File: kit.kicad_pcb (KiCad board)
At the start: 4 copper layers, 15 x 11.5 mm, 68 parts, among them IC1 TPA6130A2RTJR, J1 SJ-43617-SMT-TR, J2 Conn_01x06, U1 ESP32-S3-WROOM-1, U2 PCM5100A, U3 MIC5504-3.3YM5

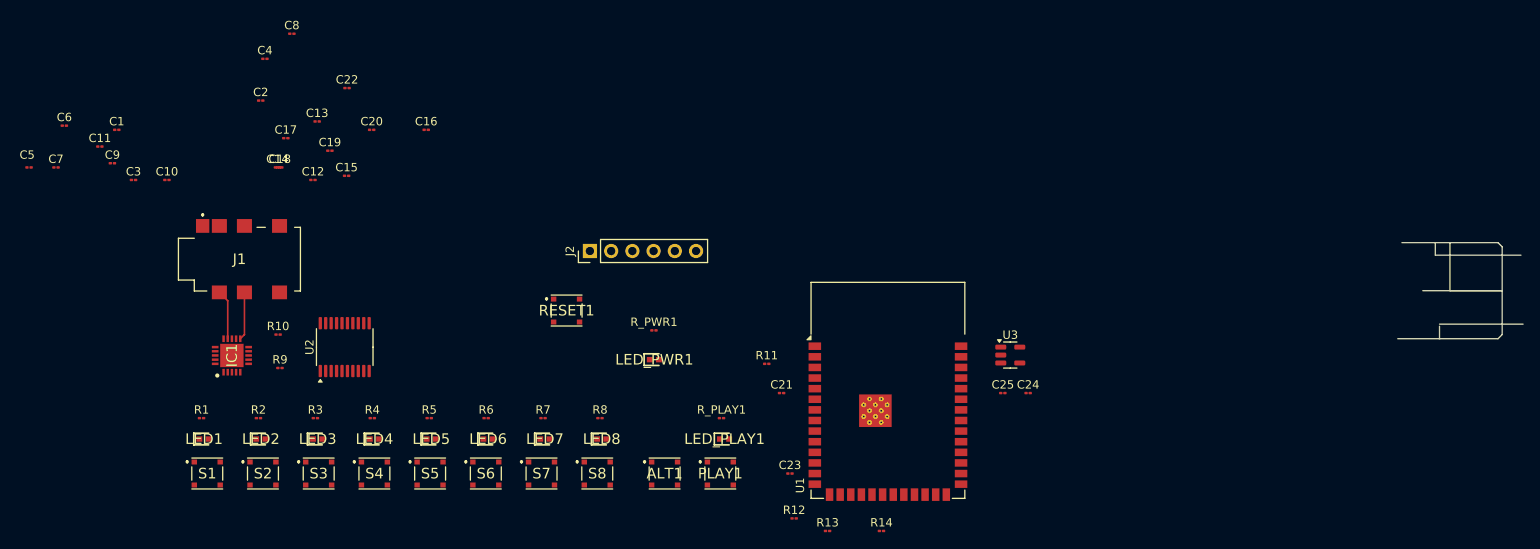
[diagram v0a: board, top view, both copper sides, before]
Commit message: Updates
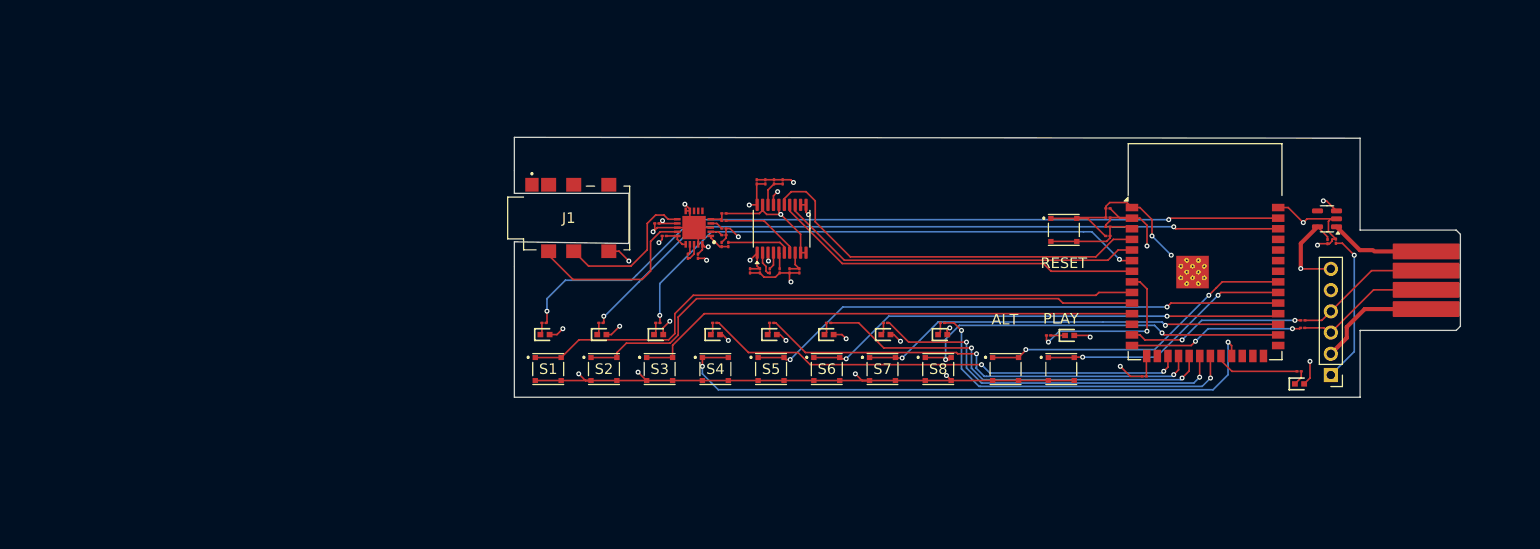
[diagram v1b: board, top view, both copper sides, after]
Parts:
- removed C11, C8: 0.47uF, Capacitor_SMD:C_01005_0402Metric
- moved C22 92.8 mm to (149.8, 40.7)
- moved J2 89.9 mm to (176.5, 57.3), turned to 180 degrees
- moved C5 80.7 mm to (100.8, 43.1), turned to -90 degrees
- moved R_PWR1 77.4 mm to (172.7, 56.9)
- moved LED_PWR1 77.3 mm to (172.8, 58.4)
- moved C6 76.2 mm to (99.6, 43.1), turned to 90 degrees
- moved C9 73.7 mm to (103.9, 40.6), turned to 180 degrees
- moved C7 72.2 mm to (95.8, 39.2), turned to 180 degrees
- moved C3 70.8 mm to (103.6, 41.7), turned to -90 degrees
- moved C10 66.9 mm to (103.9, 39.8), turned to 180 degrees
- moved C1 66.7 mm to (96.7, 40.7)
- moved C4 65.5 mm to (109.4, 44.9), turned to 90 degrees
- moved R12 65.3 mm to (173.2, 50.8)
- moved R13 61.8 mm to (173.1, 51.7)
- moved C14 60.5 mm to (110.9, 34.2), turned to -90 degrees
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- renumbered ALT1 to ALT, PLAY1 to PLAY, RESET1 to RESET
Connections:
- ALT pad 1: /SW_PLAY -> /SW_ALT
- ALT pad 3: /SW_PLAY -> /SW_ALT
- C2 pad 1: Net-(C11-Pad1) -> Net-(IC1-RIGHTINM)
- C3 pad 2: Net-(C3-Pad2) -> Net-(IC1-LEFTINM)
- J2 pad 3: /USB_DN -> /USB_DP
- J2 pad 4: /USB_DP -> /USB_DN
- PLAY pad 1: /SW_ALT -> /SW_PLAY
- PLAY pad 3: /SW_ALT -> /SW_PLAY
- R10 pad 2: Net-(C11-Pad1) -> Net-(IC1-RIGHTINM)
- R9 pad 2: Net-(C3-Pad2) -> Net-(IC1-LEFTINM)
- U1 pad 28: /SW_5 -> /SW_8
- U1 pad 29: /SW_6 -> /SW_7
- U1 pad 30: /SW_7 -> /SW_6
- U1 pad 31: /SW_8 -> /SW_5
- U1 pad 7: /LCM_DIN -> /PCM_DIN
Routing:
- net GND: track 0.00 -> 199.9 mm, vias 0 -> 19
- net +5V: track 0.00 -> 138.7 mm, vias 0 -> 4
- net /LED_1: track 0.00 -> 94.6 mm, vias 0 -> 2
- net /LED_2: track 0.00 -> 86.1 mm, vias 0 -> 2
- net /SW_1: track 0.00 -> 76.0 mm
- net /SW_4: track 0.00 -> 75.2 mm, vias 0 -> 2
- net /SW_2: track 0.00 -> 69.5 mm
- net /LED_3: track 0.00 -> 65.2 mm, vias 0 -> 2
- net /SW_5: track 0.00 -> 65.1 mm, vias 0 -> 2
- net /SW_3: track 0.00 -> 61.1 mm
- net +3.3V: track 0.00 -> 58.8 mm, vias 0 -> 16
- net /LED_4: track 0.00 -> 58.1 mm, vias 0 -> 2
- net /SW_6: track 0.00 -> 57.9 mm, vias 0 -> 2
- net /LED_5: track 0.00 -> 54.2 mm, vias 0 -> 2
- net /SW_7: track 0.00 -> 50.9 mm, vias 0 -> 2
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- added copper zone on In2.Cu, net +3.3V
- added copper zone on In1.Cu, net GND
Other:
- board size 15 x 11.5 mm -> 113.2 x 31.1 mm
- board text added: "kit pcb 06"
